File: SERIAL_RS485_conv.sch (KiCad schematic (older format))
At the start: 8 parts, among them P6 TB_IN, P7 TB_OUT, U5 ST3485EBDR, U6 ST3485EBDR

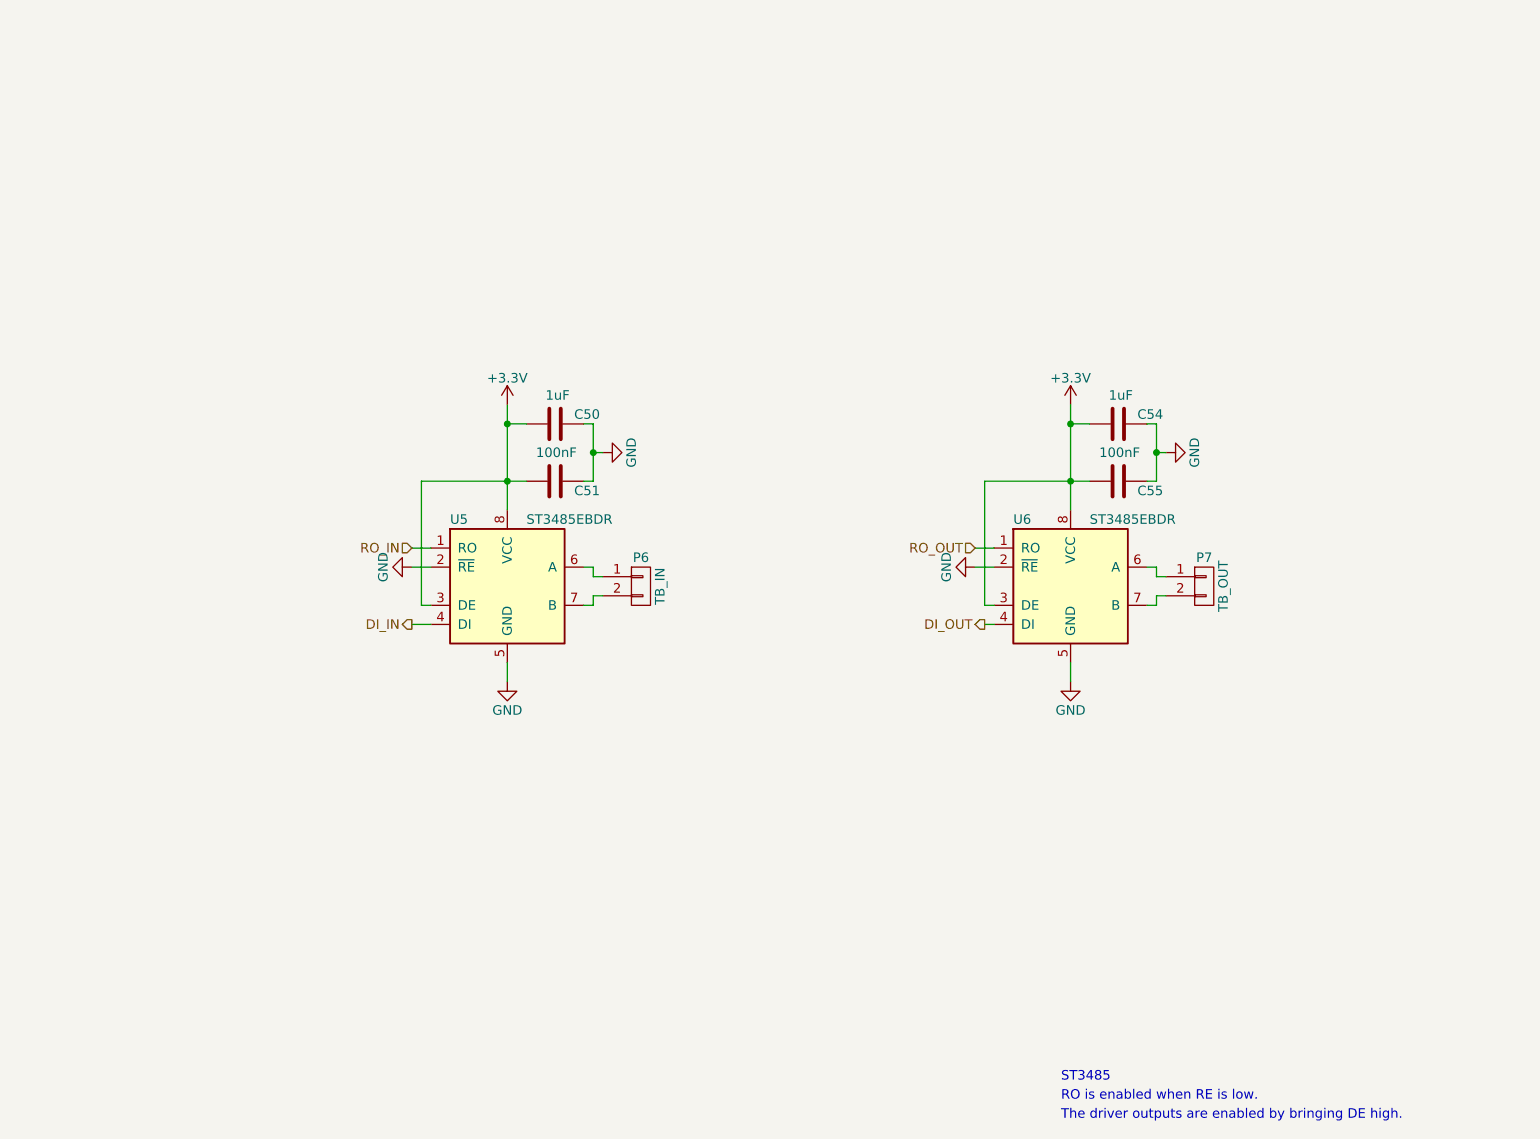
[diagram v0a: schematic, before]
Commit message: Modified schematic. v1.1
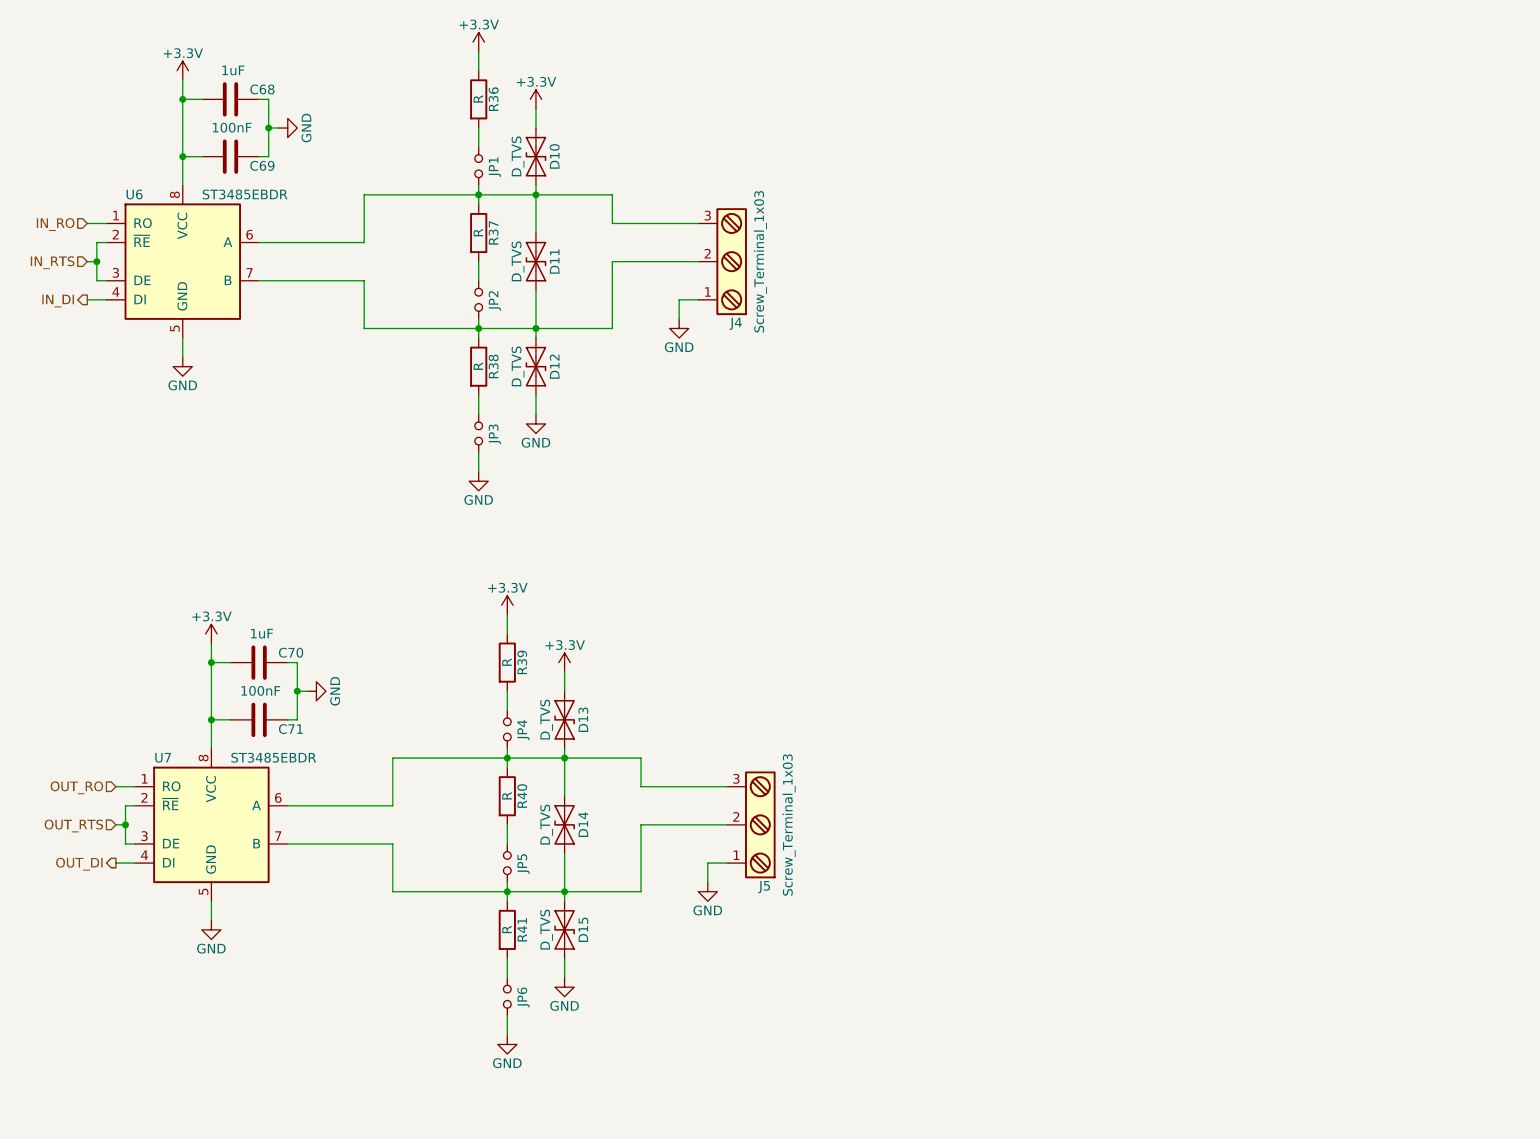
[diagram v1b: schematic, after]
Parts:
- removed P6: TB_IN, Connectors_Terminal_Blocks:TerminalBlock_Pheonix_PT-3.5mm_2pol, symbol CONN_01X02
- removed P7: TB_OUT, Connectors_Terminal_Blocks:TerminalBlock_Pheonix_PT-3.5mm_2pol, symbol CONN_01X02
- added D10, D11, D12, D13, D14, D15: D_TVS, Diodes_SMD:D_SMA-SMB_Universal_Handsoldering, symbol D_TVS
- added J4, J5: Screw_Terminal_1x03, Connectors_Terminal_Blocks:TerminalBlock_Pheonix_PT-3.5mm_3pol, symbol Screw_Terminal_1x03
- added JP1, JP2, JP3, JP4, JP5, JP6: Jumper_NO_Small, Pin_Headers:Pin_Header_Straight_1x02_Pitch2.54mm, symbol Jumper_NO_Small
- added R36, R37, R38, R39, R40, R41: R, Resistors_SMD:R_0603_HandSoldering, symbol R
- renumbered C50 to C68, C51 to C69, C54 to C70, C55 to C71, U5 to U6, U6 to U7
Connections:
- net +3V3: now also D10.1 (A1), D13.1 (A1), R36.1, R39.1; no longer U6.3 (DE), U7.3 (DE)
- net GND: now also D12.2 (A2), D15.2 (A2), J4.1, J5.1, JP3.2, JP6.2; no longer U6.2 (~RE~), U7.2 (~RE~)
- net at U6.6 (A): now also D10.2 (A2), D11.1 (A1), J4.3, JP1.2, R37.1
- net at U6.7 (B): now also D11.2 (A2), D12.1 (A1), J4.2, JP2.2, R38.1
- net at U7.6 (A): now also D13.2 (A2), D14.1 (A1), J5.3, JP4.2, R40.1
- net at U7.7 (B): now also D14.2 (A2), D15.1 (A1), J5.2, JP5.2, R41.1
- net DI_IN renamed IN_DI
- net DI_OUT renamed OUT_DI
- net RO_IN renamed IN_RO
- net RO_OUT renamed OUT_RO
- new net: JP3.1, R38.2
- new net: JP2.1, R37.2
- new net: JP1.1, R36.2
- new net: JP6.1, R41.2
- new net: JP5.1, R40.2
- new net: JP4.1, R39.2
- new net IN_RTS: U6.2 (~RE~), U6.3 (DE)
- new net OUT_RTS: U7.2 (~RE~), U7.3 (DE)
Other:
- note removed: "RO is enabled when RE is low."
- note removed: "ST3485"
- note removed: "The driver outputs are enabled by bringing DE high."
- moved on the sheet: C68, C69, C70, C71, U6, U7
